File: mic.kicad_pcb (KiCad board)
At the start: 2 copper layers, 50 x 50 mm, 38 parts, among them J1 AudioPlug3, J2 USB_C_Receptacle_USB2.0_16P, SW1 SW_Push, U1 TS5A3159ADBVR, U2 INA826AID, U3 PCM2902CDBR, U4 TLV70033_SOT23-5, Y1 12MHz

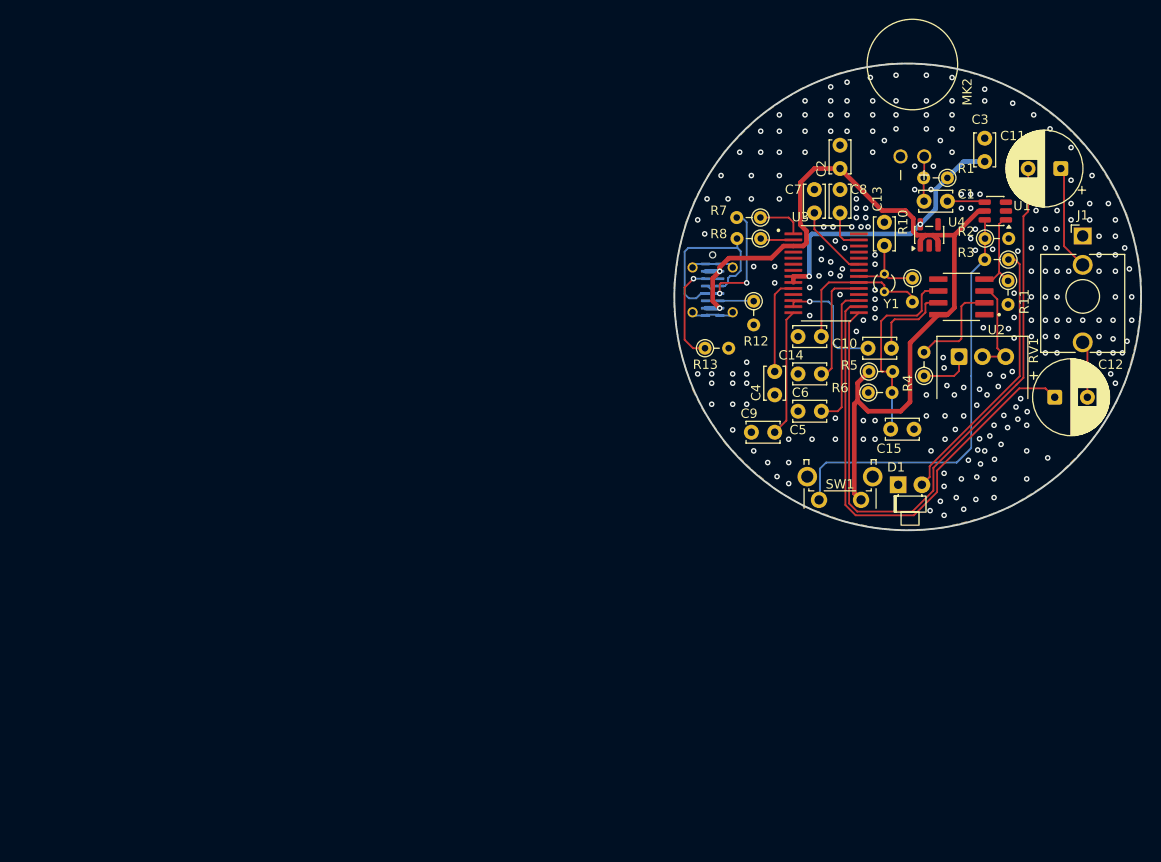
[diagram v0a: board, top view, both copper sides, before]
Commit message: alternative version
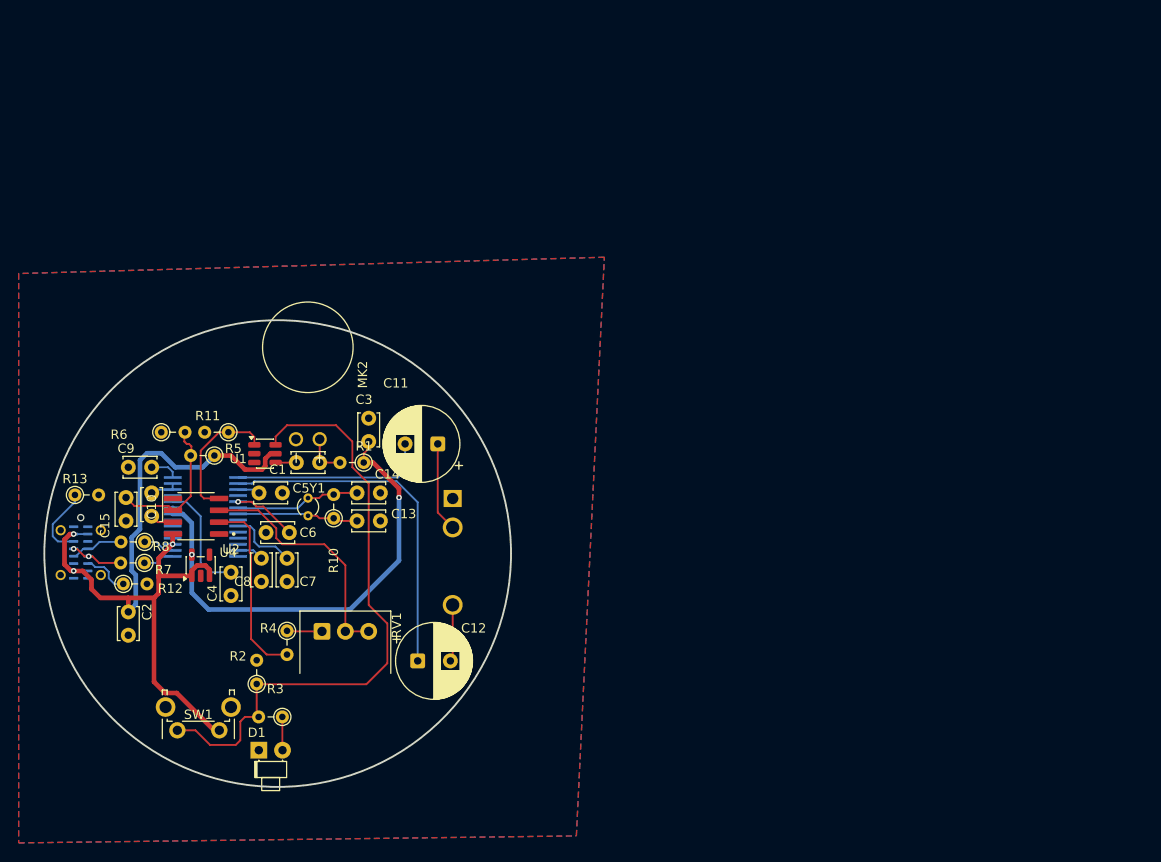
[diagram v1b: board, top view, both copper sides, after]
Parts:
- J1, U3: moved to B.Cu
- moved C2 92.6 mm to (84.0, 108.8), turned to 90 degrees
- moved R3 91.9 mm to (100.5, 117.5)
- moved R2 91.5 mm to (97.8, 114.0), turned to 90 degrees
- moved U4 85.7 mm to (91.8, 101.2)
- moved U2 85.3 mm to (91.2, 96.0)
- moved R11 85.1 mm to (94.7, 87.0), turned to 180 degrees
- moved C15 85.0 mm to (83.8, 96.5), turned to 90 degrees
- moved U1 82.5 mm to (98.6, 89.3), turned to 0 degrees
- moved C10 78.3 mm to (86.5, 93.5), turned to -90 degrees
- moved R6 75.9 mm to (87.5, 87.0)
- moved R7 75.7 mm to (85.7, 101.0)
- moved C8 74.9 mm to (98.2, 103.0), turned to 90 degrees
- moved RV1 74.3 mm to (104.8, 108.3)
- moved D1 74.2 mm to (98.0, 121.1)
- moved R12 74.0 mm to (83.5, 103.2), turned to 0 degrees
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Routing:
- net Net-(U3-VOUTR): track 69.9 -> 21.1 mm
- net Net-(D1-A): track 29.4 -> 3.57 mm
- net +3.3V: track 29.9 -> 50.8 mm, vias 3 -> 2
- net Net-(R2-Pad1): track 45.6 -> 66.4 mm
- net Net-(U2-RG_3): track 10.8 -> 26.2 mm
- net Net-(U3-VOUTL): track 52.7 -> 37.3 mm
- net Net-(J2-D--PadA7): track 19.8 -> 5.70 mm
- net Net-(U3-VCCP1I): track 15.4 -> 2.38 mm
- net Net-(U3-VCOM): track 13.6 -> 3.06 mm
- net Net-(U3-VINL): track 13.1 -> 3.04 mm, vias 1 -> 0
- net Earth: track 9.59 -> 0.00 mm, vias 233 -> 0
- net Net-(U2-RG_2): track 10.7 -> 20.0 mm
- net Net-(J2-D+-PadA6): track 13.6 -> 5.67 mm
- net +5V: track 94.7 -> 88.0 mm, vias 2 -> 3
- net Net-(U2-VOUT): track 9.19 -> 2.54 mm
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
